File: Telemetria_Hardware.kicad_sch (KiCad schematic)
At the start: 27 parts, among them M100A1 1715734, SW1 RESET BUTTON, U1 CA3140, U2 CA3140

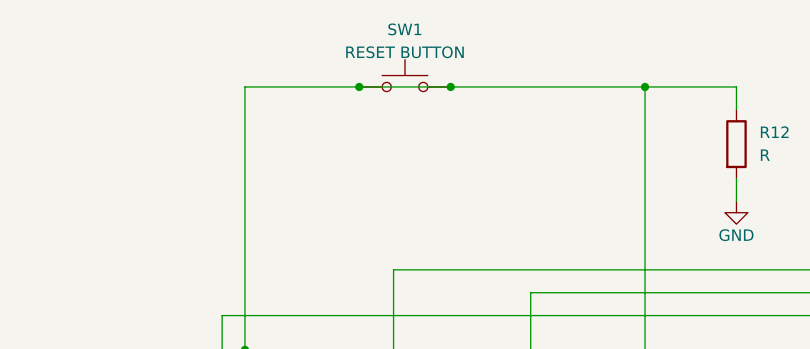
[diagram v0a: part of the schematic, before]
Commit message: upp
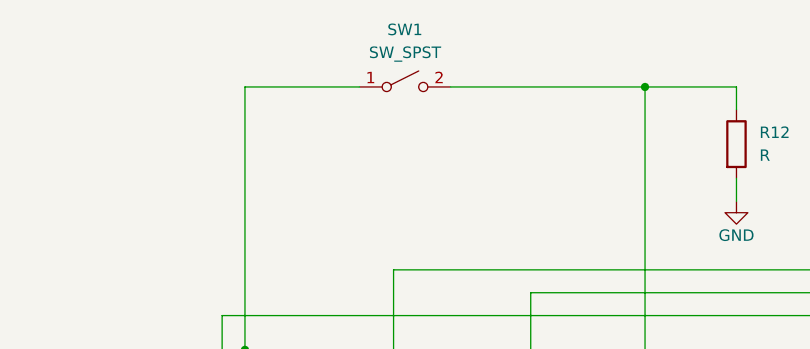
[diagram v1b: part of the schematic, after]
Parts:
- removed SW1: RESET BUTTON, BUTT:BUTT, symbol Switch:SW_MEC_5G
- added SW1: SW_SPST, Button_Switch_THT:SW_DIP_SPSTx01_Slide_9.78x4.72mm_W7.62mm_P2.54mm, symbol Switch:SW_SPST
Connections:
- net at ADS1115.1 (VDD), ESP32.16 (3V3): now also SW1.1 (A); no longer ESP32.20 (IO4), R12.1
- new net: ESP32.20 (IO4), R12.1, SW1.2 (B)
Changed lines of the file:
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@@
 	)
 	(junction
-		(at 60.96 22.86)
-		(diameter 0)
-		(color 0 0 0 0)
-	)
-	(junction
 		(at 127 110.49)
 		(diameter 0)
@@
 	)
 	(junction
-		(at 50.8 22.86)
-		(diameter 0)
-		(color 0 0 0 0)
-	)
-	(junction
 		(at 127 137.16)
 		(diameter 0)
@@
 	(wire
 		(pts
-			(xy 50.8 22.86) (xy 60.96 22.86)
-		)
-		(stroke
-			(width 0)
-			(type default)
-		)
-	)
-	(wire
-		(pts
 			(xy 227.33 82.55) (xy 233.68 82.55)
 		)
@@
 	)
 	(symbol
-		(lib_id "Switch:SW_MEC_5G")
-		(at 55.88 22.86 0)
-		(unit 1)
-		(exclude_from_sim no)
-		(in_bom yes)
-		(on_board yes)
-		(dnp no)
-		(property "Reference" "SW1"
-			(at 55.88 16.51 0)
-			(effects
-				(font
-					(size 1.27 1.27)
-				)
-			)
-		)
-		(property "Value" "RESET BUTTON"
-			(at 55.88 19.05 0)
-			(effects
-				(font
-					(size 1.27 1.27)
-				)
-			)
-		)
-		(property "Footprint" "BUTT:BUTT"
-			(at 55.88 17.78 0)
-			(effects
-				(font
-					(size 1.27 1.27)
-				)
-				(hide yes)
-			)
-		)
-		(property "Datasheet" "http://www.apem.com/int/index.php?controller=attachment&id_attachment=488"
-			(at 55.88 17.78 0)
-			(effects
-				(font
-					(size 1.27 1.27)
-				)
-				(hide yes)
-			)
-		)
-		(property "Description" ""
-			(at 55.88 22.86 0)
-			(effects
-				(font
-					(size 1.27 1.27)
-				)
-				(hide yes)
-			)
-		)
-		(pin "1"
-		)
-		(pin "2"
-		)
-		(pin "4"
-		)
-		(pin "3"
-		)
-		(instances
-			(project "Telemetria_Hardware"
-				(path "/c806ca64-4076-499b-9029-155759542c55"
-					(reference "SW1")
-					(unit 1)
-				)
-			)
-		)
-	)
-	(symbol
 		(lib_id "Amplifier_Operational:CA3140")
 		(at 251.46 43.18 180)
@@
 					(unit 1)
 				)
+			)
+		)
+	)
+	(symbol
+		(lib_id "Switch:SW_SPST")
+		(at 55.88 22.86 0)
+		(unit 1)
+		(exclude_from_sim no)
+		(in_bom yes)
+		(on_board yes)
+		(dnp no)
+		(fields_autoplaced yes)
+		(property "Reference" "SW1"
+			(at 55.88 16.51 0)
+			(effects
+				(font
+					(size 1.27 1.27)
+				)
+			)
+		)
+		(property "Value" "SW_SPST"
+			(at 55.88 19.05 0)
+			(effects
+				(font
+					(size 1.27 1.27)
+				)
+			)
+		)
+		(property "Footprint" "Button_Switch_THT:SW_DIP_SPSTx01_Slide_9.78x4.72mm_W7.62mm_P2.54mm"
+			(at 55.88 22.86 0)
+			(effects
+				(font
+					(size 1.27 1.27)
+				)
+				(hide yes)
+			)
+		)
+		(property "Datasheet" "~"
+			(at 55.88 22.86 0)
+			(effects
+				(font
+					(size 1.27 1.27)
+				)
+				(hide yes)
+			)
+		)
+		(property "Description" "Single Pole Single Throw (SPST) switch"
+			(at 55.88 22.86 0)
+			(effects
+				(font
+					(size 1.27 1.27)
+				)
+				(hide yes)
+			)
+		)
+		(pin "2"
+		)
+		(pin "1"
+		)
+		(instances
+			(project "Telemetria_Hardware"
+				(path "/c806ca64-4076-499b-9029-155759542c55"
+					(reference "SW1")
+					(unit 1)
+				)
